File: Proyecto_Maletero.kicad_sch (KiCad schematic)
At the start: 44 parts, among them J2 Conn_01x02, J3 Conn_01x02, J4 Conn_01x03, J5 Conn_01x02, J7 Conn_01x03, J8 Conn_01x02, J9 Conn_01x02, SW1 SW_Push, SW3 SW_SPST, U1 LT1117-ADJ, U2 MCP2551-I-SN, U3 PIC18F258-I_SO, U4 L298HN, U5 LM321, Y1 4MHz

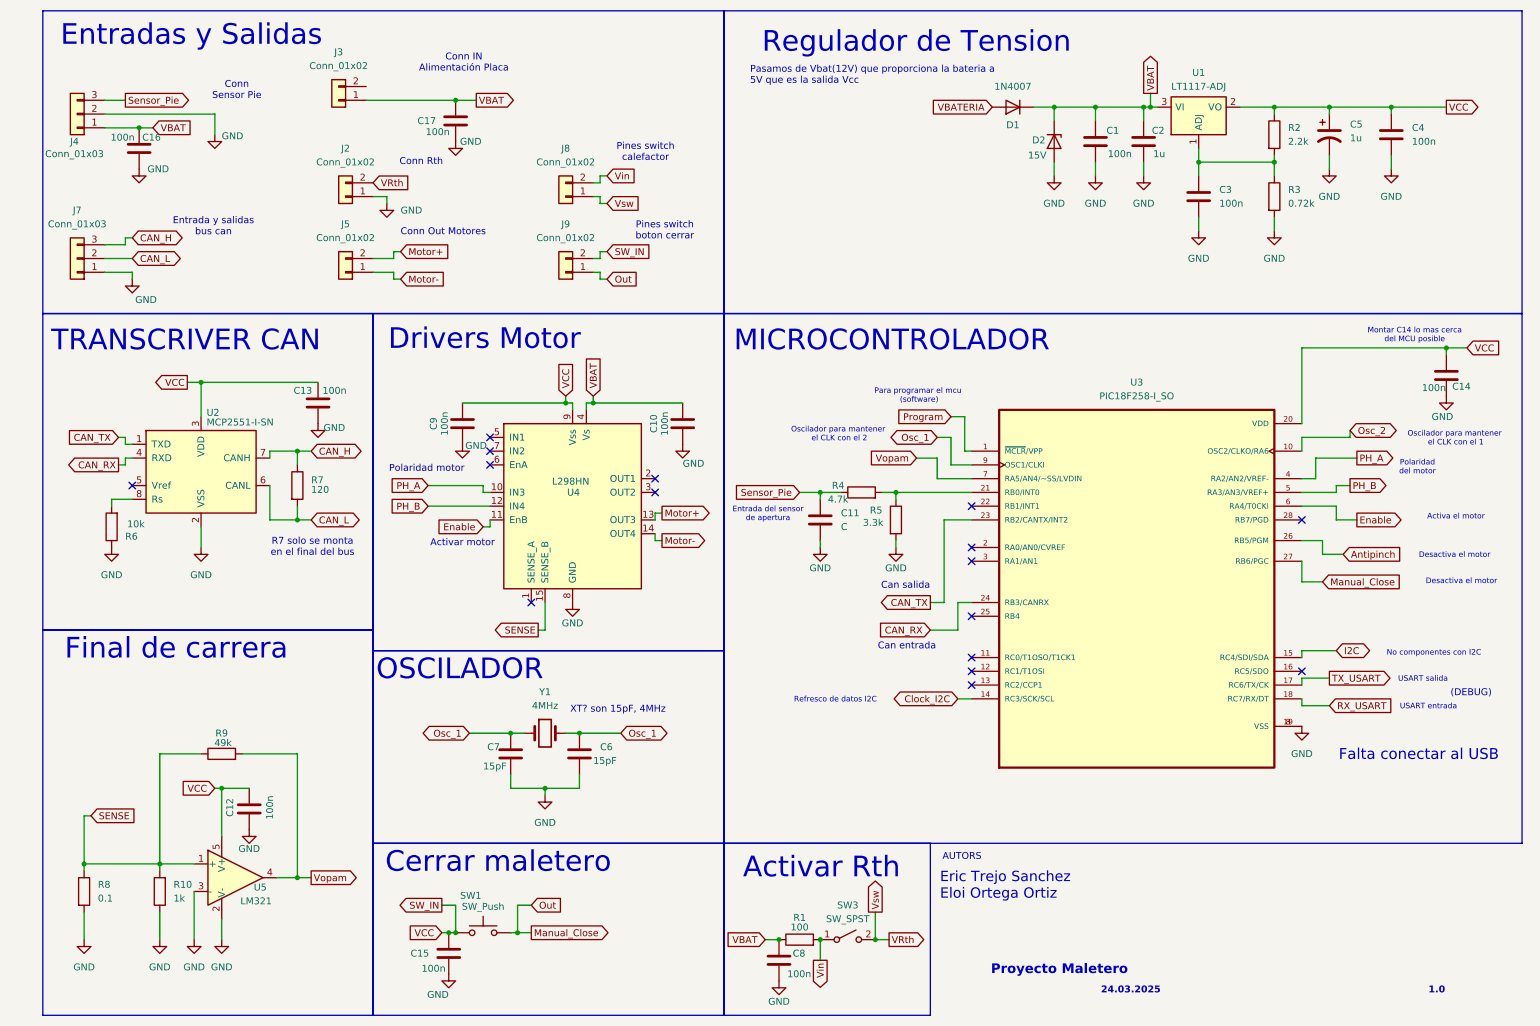
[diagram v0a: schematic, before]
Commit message: Rth menos enano
Hemos expandido Rth
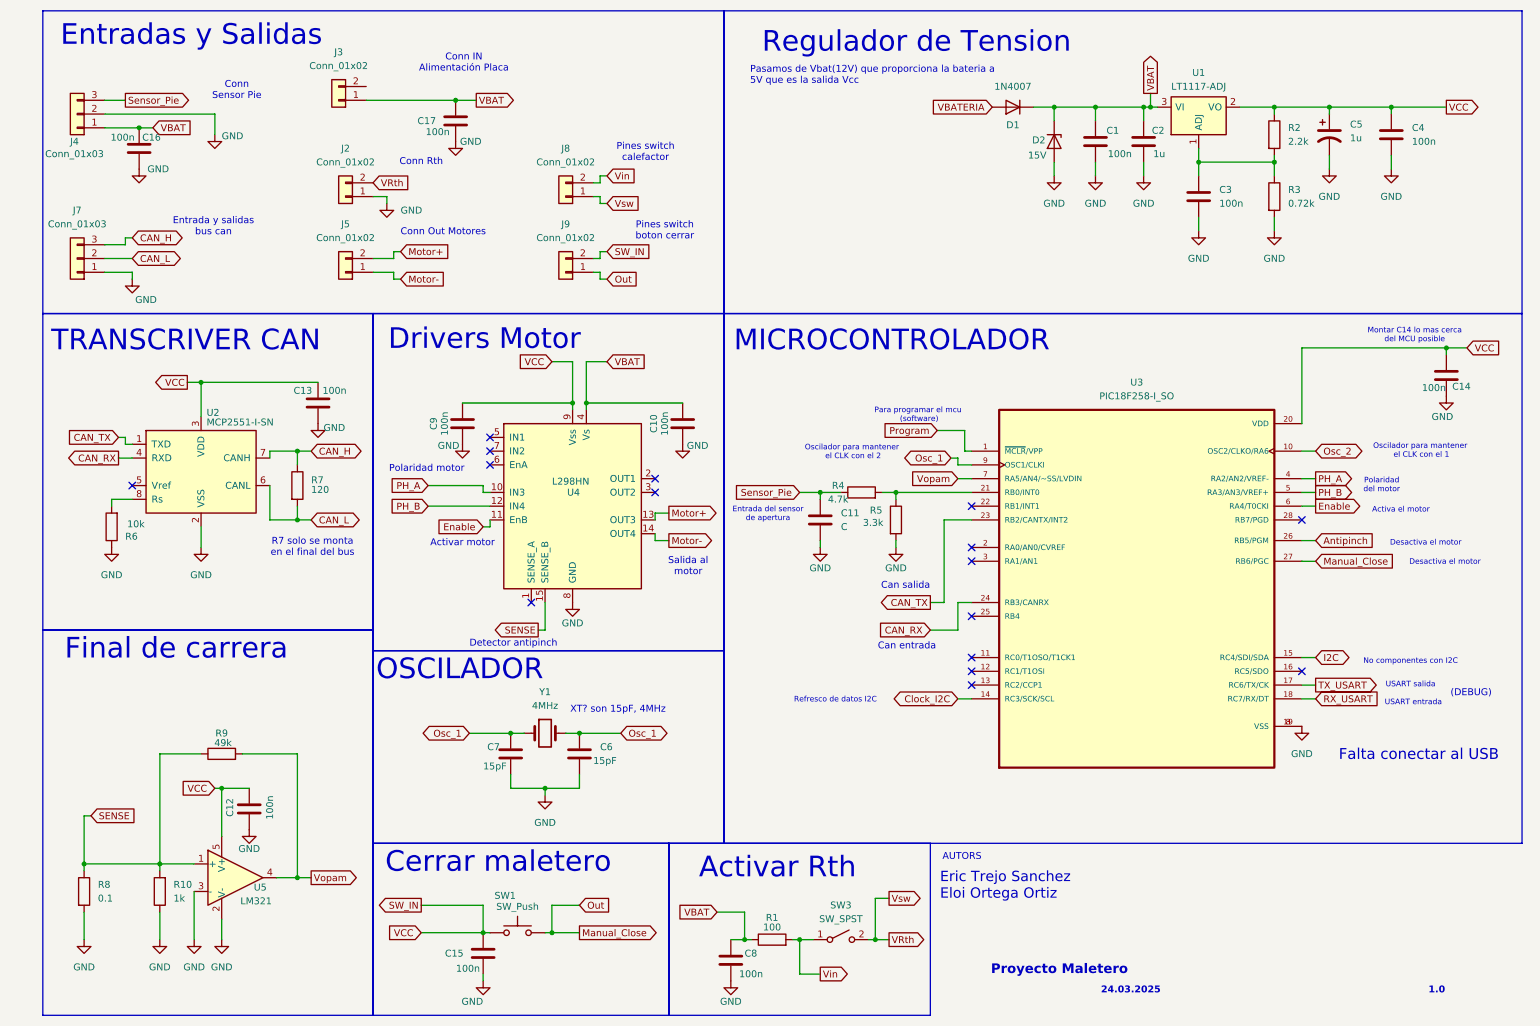
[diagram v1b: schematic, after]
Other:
- note added: "Detector antipinch"
- note added: "Salida al motor"
- moved on the sheet: C15, C8, R1, SW1, SW3
